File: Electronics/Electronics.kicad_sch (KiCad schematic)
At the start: 44 parts, among them J1 Raspberry_Pi_2_3, J10 USB_C_Receptacle_PowerOnly_6P, J11 FAN_OUT, J12 DIAL, J2 HANDSET, J3 EXT_ADC, J4 USB-C_PD_IN, J5 USB-C_PD_OUT, J6 HOOK_SWITCH_TERM, J9 RINGER_BELL, Q1 AO3400A, U1 DRV8871DDA, U2 MT3608, U3 MAX98357A, U4 IP2721

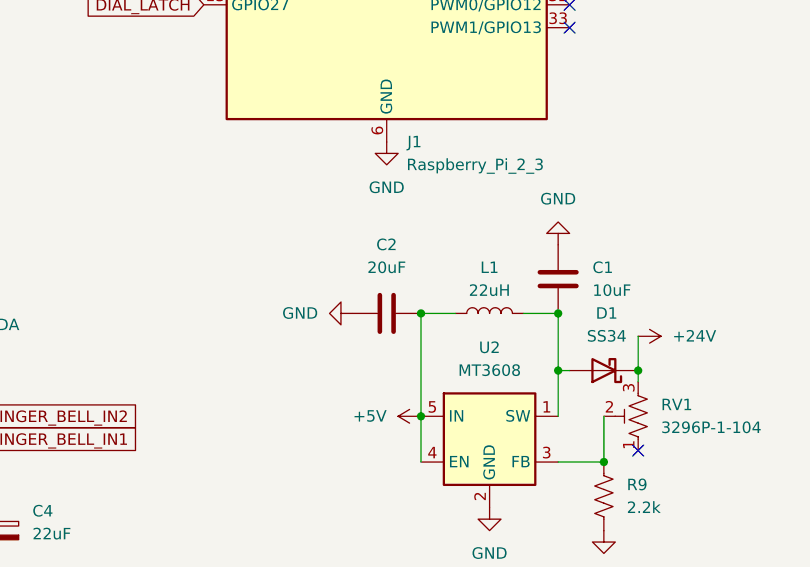
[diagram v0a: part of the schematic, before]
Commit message: Finalized production exports and now awaiting PCBs to arrive
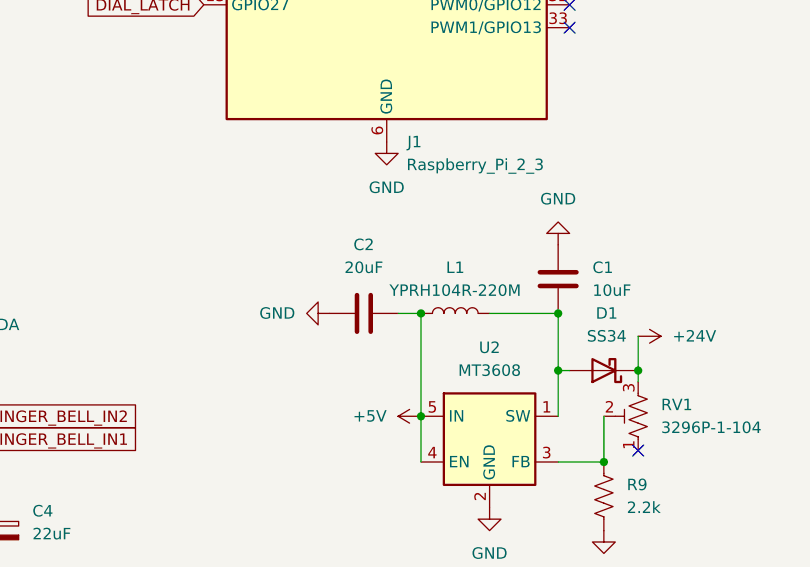
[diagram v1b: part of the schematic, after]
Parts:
- L1: value 22uH -> YPRH104R-220M; footprint AdditionalComponents:CYL104R-22UH -> AdditionalComponents:YPRH104R-220M
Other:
- moved on the sheet: C2, L1
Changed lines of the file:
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@@
+	(wire
+		(pts
+			(xy 207.01 130.81) (xy 209.55 130.81)
+		)
+		(stroke
+			(width 0)
+			(type default)
+		)
+	)
 	(wire
 		(pts
@@
 	(wire
 		(pts
-			(xy 224.79 130.81) (xy 220.98 130.81)
-		)
-		(stroke
-			(width 0)
-			(type default)
-		)
-	)
-	(wire
-		(pts
-			(xy 209.55 130.81) (xy 213.36 130.81)
+			(xy 224.79 130.81) (xy 217.17 130.81)
 		)
 		(stroke
@@
 	(symbol
 		(lib_id "power:GND")
-		(at 201.93 130.81 270)
+		(at 199.39 130.81 270)
 		(unit 1)
 		(exclude_from_sim no)
@@
 		(dnp no)
 		(property "Reference" "#PWR017"
-			(at 195.58 130.81 0)
+			(at 193.04 130.81 0)
 			(effects
 				(font
@@
 		)
 		(property "Value" "GND"
-			(at 198.12 130.8101 90)
+			(at 195.58 130.8101 90)
 			(effects
 				(font
@@
 		)
 		(property "Footprint" ""
-			(at 201.93 130.81 0)
+			(at 199.39 130.81 0)
 			(effects
 				(font
@@
 		)
 		(property "Datasheet" ""
-			(at 201.93 130.81 0)
+			(at 199.39 130.81 0)
 			(effects
 				(font
@@
 		)
 		(property "Description" "Power symbol creates a global label with name \"GND\" , ground"
-			(at 201.93 130.81 0)
+			(at 199.39 130.81 0)
 			(effects
 				(font
@@
 	(symbol
 		(lib_id "Device:C")
-		(at 205.74 130.81 270)
+		(at 203.2 130.81 270)
 		(unit 1)
 		(exclude_from_sim no)
@@
 		(fields_autoplaced yes)
 		(property "Reference" "C2"
-			(at 205.74 123.19 90)
+			(at 203.2 123.19 90)
 			(effects
 				(font
@@
 		)
 		(property "Value" "20uF"
-			(at 205.74 125.73 90)
+			(at 203.2 125.73 90)
 			(effects
 				(font
@@
 		)
 		(property "Footprint" "Capacitor_SMD:C_0603_1608Metric"
-			(at 201.93 131.7752 0)
+			(at 199.39 131.7752 0)
 			(effects
 				(font
@@
 		)
 		(property "Datasheet" "~"
-			(at 205.74 130.81 0)
+			(at 203.2 130.81 0)
 			(effects
 				(font
@@
 		)
 		(property "Description" "Unpolarized capacitor"
-			(at 205.74 130.81 0)
+			(at 203.2 130.81 0)
 			(effects
 				(font
@@
 	(symbol
 		(lib_id "Device:L")
-		(at 217.17 130.81 90)
+		(at 213.36 130.81 90)
 		(unit 1)
 		(exclude_from_sim no)
@@
 		(fields_autoplaced yes)
 		(property "Reference" "L1"
-			(at 217.17 125.73 90)
-			(effects
-				(font
-					(size 1.27 1.27)
-				)
-			)
-		)
-		(property "Value" "22uH"
-			(at 217.17 128.27 90)
-			(effects
-				(font
-					(size 1.27 1.27)
-				)
-			)
-		)
-		(property "Footprint" "AdditionalComponents:CYL104R-22UH"
-			(at 217.17 130.81 0)
+			(at 213.36 125.73 90)
+			(effects
+				(font
+					(size 1.27 1.27)
+				)
+			)
+		)
+		(property "Value" "YPRH104R-220M"
+			(at 213.36 128.27 90)
+			(effects
+				(font
+					(size 1.27 1.27)
+				)
+			)
+		)
+		(property "Footprint" "AdditionalComponents:YPRH104R-220M"
+			(at 213.36 130.81 0)
 			(effects
 				(font
@@
 		)
 		(property "Datasheet" "~"
-			(at 217.17 130.81 0)
+			(at 213.36 130.81 0)
 			(effects
 				(font
@@
 		)
 		(property "Description" "Inductor"
-			(at 217.17 130.81 0)
-			(effects
-				(font
+			(at 213.36 130.81 0)
+			(effects
+				(font
